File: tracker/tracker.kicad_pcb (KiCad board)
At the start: 2 copper layers, 50.5 x 56.9 mm, 76 parts, among them J1 Conn_01x10, J2 SIM_Card, M1 BG96, Q1 SSM6N7002KFU, Q2 SSM6N7002KFU, Q3 SSM6N7002KFU, U1 STM32U545CEUx, U2 GD25QxxxEY, U3 74LVC244APW,118, U4 AP22800HB-7, U5 DF5A6.8JE,LM, U6 LMR51430, U7 AP61100Z6, U8 BQ25601, Y1 32.768KHz, Y2 8MHz

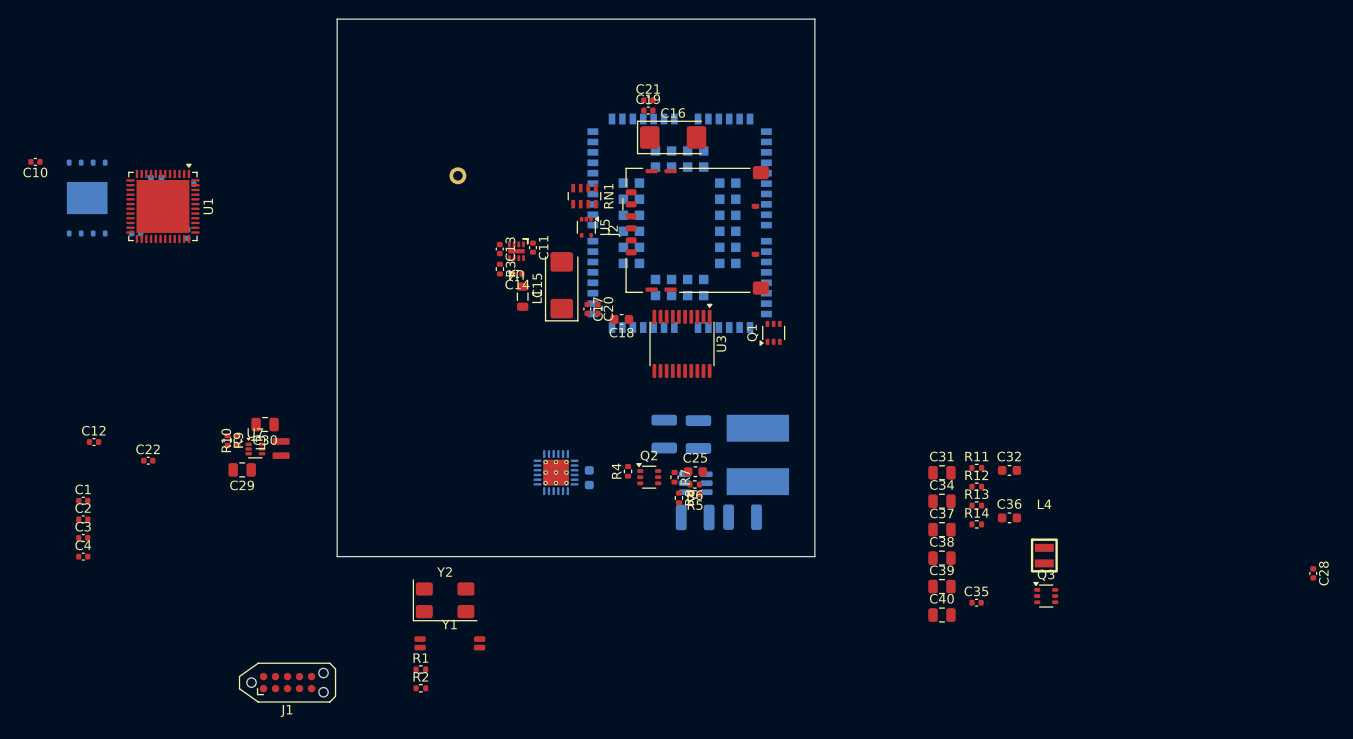
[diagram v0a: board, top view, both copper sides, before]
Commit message: save
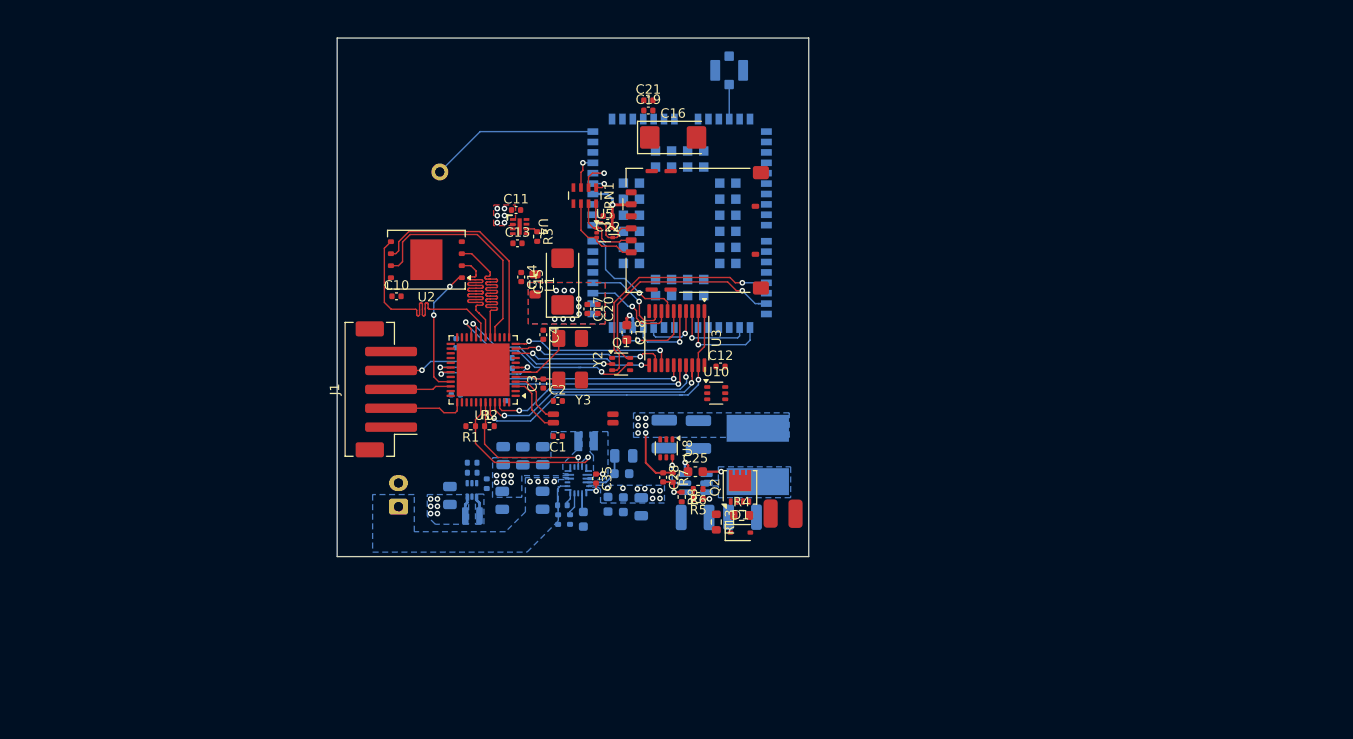
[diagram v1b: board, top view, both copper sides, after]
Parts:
- removed C34: 10u, Capacitor_SMD:C_0805_2012Metric
- removed Q3: SSM6N7002KFU, Package_TO_SOT_SMD:SOT-363_SC-70-6
- removed Y1: 32.768KHz, Crystal:Crystal_SMD_SeikoEpson_MC146-4Pin_6.7x1.5mm
- added C41: 10u, Capacitor_SMD:C_0805_2012Metric, B.Cu at (152.9, 87.2)
- added C42: 0.1u, Capacitor_SMD:C_0603_1608Metric, B.Cu at (152.7, 89.1)
- added D1: 12V, Diode_SMD:D_SOD-323, F.Cu at (165.2, 95.3)
- added J3: Conn_01x01, My Footprints:pad_smd_1.5x3, F.Cu at (168.4, 93.3)
- added J4: Conn_01x01, My Footprints:pad_smd_1.5x3, F.Cu at (171.1, 93.3)
- added J5: Conn_Coaxial, Connector_Coaxial:U.FL_Molex_MCRF_73412-0110_Vertical, B.Cu at (164.0, 46.4)
- added J6: Conn_01x02, Connector_JST:JST_XH_B2B-XH-A_1x02_P2.50mm_Vertical, B.Cu at (129.0, 92.6)
- added R15: TBD, Resistor_SMD:R_0402_1005Metric, B.Cu at (147.2, 94.0)
- added U10: PUMH10,115, Package_TO_SOT_SMD:SOT-363_SC-70-6, F.Cu at (162.7, 80.6)
- added U9: ~, My Footprints:BQ25622E, B.Cu at (148.1, 89.8)
- added Y3: 32.768KHz, Crystal:Crystal_SMD_SeikoEpson_MC146-4Pin_6.7x1.5mm, F.Cu at (148.6, 83.3)
- C29, C30, C31, C32, C36, C37, C38, C39, C40, L3, L4, R10, R11, R12, R9, U7: moved to B.Cu
- J1: value Conn_01x10 -> Conn_01x05; footprint Connector:Tag-Connect_TC2050-IDC-NL_2x05_P1.27mm_Vertical -> Connector_JST:JST_PH_B5B-PH-SM4-TB_1x05-1MP_P2.00mm_Vertical
- Q2: value SSM6N7002KFU -> DMP2008UFG; footprint Package_TO_SOT_SMD:SOT-363_SC-70-6 -> Package_SON:Diodes_PowerDI3333-8
- R13: value 37K -> 10K; footprint Resistor_SMD:R_0402_1005Metric -> Resistor_SMD:R_0603_1608Metric
- R14: value 100K -> 200K; moved to B.Cu
- R4: value 200K -> 220K; footprint Resistor_SMD:R_0402_1005Metric -> Resistor_SMD:R_0603_1608Metric
- U2: moved to F.Cu
- U8: value BQ25601 -> PUMH10,115; footprint Package_DFN_QFN:Texas_RTW_WQFN-24-1EP_4x4mm_P0.5mm_EP2.7x2.7mm_ThermalVias -> Package_TO_SOT_SMD:SOT-363_SC-70-6; moved to F.Cu
- moved C28 69.5 mm to (157.0, 89.5)
- moved C12 66.8 mm to (163.1, 77.8)
- moved C22 55.1 mm to (151.2, 61.8), turned to 180 degrees
- moved C4 54.0 mm to (144.4, 74.4), turned to -90 degrees
- moved R14 52.0 mm to (138.4, 90.2), turned to 90 degrees
- moved C2 51.8 mm to (145.9, 81.4)
- moved C3 51.4 mm to (144.4, 79.6), turned to 90 degrees
- moved C1 50.7 mm to (145.9, 85.1), turned to 180 degrees
- moved C40 49.4 mm to (140.1, 87.2), turned to 90 degrees
- moved L4 49.0 mm to (149.7, 85.7), turned to 90 degrees
- moved C39 46.5 mm to (142.2, 87.2), turned to 90 degrees
- moved C36 45.1 mm to (148.6, 93.9), turned to -90 degrees
- moved R12 44.4 mm to (145.9, 94.0), turned to -90 degrees
- moved R11 44.0 mm to (146.4, 92.4), turned to 180 degrees
- moved C38 43.6 mm to (144.3, 87.2), turned to 90 degrees
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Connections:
- net Net-(AE1-A) renamed /gsm/ANT_GNSS
- C10 pad 1: Net-(U2-VCC) -> +3V3
- C23 pad 1: /psu/+VIN -> /psu/+VIN_PROTECTED
- C24 pad 1: /psu/+VIN -> /psu/+VIN_PROTECTED
- C29 pad 1: /low_voltage_psu/+VSYS -> +VSYS
- C30 pad 1: /low_voltage_psu/+3V3 -> +3V3
- C35 pad 2: Net-(U8-BTST) -> Net-(U9-BTST)
- C36 pad 1: Net-(U8-REGN) -> Net-(U9-REGN)
- C37 pad 1: Net-(C37-Pad1) -> /battery charger/+BAT
- C38 pad 1: /battery charger/+VSYS -> +VSYS
- C39 pad 1: /battery charger/+VSYS -> +VSYS
- C40 pad 1: /battery charger/+VSYS -> +VSYS
- J1 pad 5: unconnected-(J1-Pin_5-Pad5) -> GND
- L3 pad 2: /low_voltage_psu/+3V3 -> +3V3
- L4 pad 2: /battery charger/+VSYS -> +VSYS
- M1 pad 60: unconnected-(M1-ANT_MAIN-Pad60) -> /gsm/ANT_MAIN
- Q2 pad 1: /mcu/PSU_CTRL -> /psu/+VIN_PROTECTED
- Q2 pad 2: +3V3 -> /psu/+VIN_PROTECTED
- Q2 pad 3: unconnected-(Q2B-D-Pad3) -> /psu/+VIN_PROTECTED
- Q2 pad 4: unconnected-(Q2B-S-Pad4) -> Net-(D1-A)
- Q2 pad 5: unconnected-(Q2B-G-Pad5) -> /+VIN
- R11 pad 1: Net-(U8-REGN) -> Net-(U9-TS_BIAS)
- R11 pad 2: Net-(U8-TS) -> Net-(U9-TS)
- R12 pad 1: Net-(U8-TS) -> Net-(U9-TS)
- R13 pad 1: Net-(C37-Pad1) -> Net-(D1-A)
- R13 pad 2: /battery charger/BAT_LEVEL -> GND
- R14 pad 1: /battery charger/BAT_LEVEL -> /battery charger/CHARGER_PG
- R14 pad 2: GND -> +VSYS
- R4 pad 1: +3V3 -> /psu/+VIN_PROTECTED
- R4 pad 2: /mcu/PSU_CTRL -> Net-(D1-A)
- R5 pad 1: /psu/+VIN -> /psu/+VIN_PROTECTED
- R5 pad 2: Net-(Q2A-D) -> Net-(U6-EN)
- R6 pad 2: Net-(Q2A-D) -> Net-(U6-EN)
- R9 pad 2: /low_voltage_psu/+3V3 -> +3V3
- RN1 pad 1: /gsm/SIM_CLK -> /gsm/SIM_RST
- RN1 pad 3: /gsm/SIM_RST -> /gsm/SIM_CLK
- RN1 pad 6: Net-(J2-RST) -> Net-(J2-CLK)
- RN1 pad 8: Net-(J2-CLK) -> Net-(J2-RST)
- U1 pad 14: /mcu/OCTOSPI1_NCS -> unconnected-(U1-PA4-Pad14)
- U1 pad 20: unconnected-(U1-PB2-Pad20) -> /gsm/GSM_RESET
- U1 pad 21: unconnected-(U1-PB10-Pad21) -> /gsm/GSM_PWRKEY
- U1 pad 29: /gsm/GSM_STATUS -> unconnected-(U1-PA8-Pad29)
- U1 pad 33: unconnected-(U1-PA12-Pad33) -> /mcu/OCTOSPI1_NCS
- U1 pad 34: unconnected-(U1-PA13-Pad34) -> /mcu/SWDIO
- U1 pad 37: unconnected-(U1-PA14-Pad37) -> /mcu/SWCLK
- U1 pad 42: unconnected-(U1-PB6-Pad42) -> /mcu/I2C_SCL
- U1 pad 43: unconnected-(U1-PB7-Pad43) -> /mcu/I2C_SDA
- U1 pad 44: unconnected-(U1-PH3-Pad44) -> /gsm/GSM_LINE_BUF_EN
- U1 pad 45: unconnected-(U1-PB8-Pad45) -> /gsm/GSM_AP_READY
- U1 pad 46: unconnected-(U1-PB9-Pad46) -> /gsm/GSM_STATUS
- U2 pad 8: Net-(U2-VCC) -> +3V3
- U3 pad 1: (no net) -> /gsm/GSM_LINE_BUF_EN
- U6 pad 3: /psu/+VIN -> /psu/+VIN_PROTECTED
- U6 pad 5: Net-(Q2A-D) -> Net-(U6-EN)
- U7 pad 3: /low_voltage_psu/+VSYS -> +VSYS
- U7 pad 5: /low_voltage_psu/+VSYS -> /battery charger/CHARGER_PG
- U7 pad 6: /low_voltage_psu/+3V3 -> +3V3
- U8 pad 1: +5V -> /mcu/PSU_CTRL
- U8 pad 2: GND -> +3V3
- U8 pad 3: /battery charger/CHARGER_PG -> unconnected-(U8-Pad3)
- U8 pad 4: /battery charger/CHARGER_STAT -> unconnected-(U8-Pad4)
- U8 pad 5: /battery charger/CHARGER_SCL -> unconnected-(U8-Pad5)
- U8 pad 6: /battery charger/CHARGER_SDA -> Net-(U6-EN)
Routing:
- net /gsm/GSM_LINE_BUF_EN: track 0.00 -> 33.5 mm, vias 0 -> 2
- net /gsm/GPS_TX: track 0.00 -> 28.6 mm, vias 0 -> 2
- net /gsm/GPS_RX: track 0.00 -> 27.8 mm, vias 0 -> 2
- net /gsm/GSM_AP_READY: track 0.00 -> 26.6 mm, vias 0 -> 2
- net /gsm/PWRKEY: track 0.00 -> 25.4 mm, vias 0 -> 1
- net /gsm/RESET: track 0.00 -> 25.0 mm, vias 0 -> 1
- net /mcu/OCTOSPI1_IO0: track 0.00 -> 24.3 mm
- net /mcu/OCTOSPI1_IO2: track 0.00 -> 24.1 mm
- net /mcu/OCTOSPI1_IO1: track 0.00 -> 24.1 mm
- net /mcu/OCTOSPI1_IO3: track 0.00 -> 24.1 mm
- net /gsm/GSM_STATUS: track 0.00 -> 23.6 mm, vias 0 -> 2
- net /mcu/OCTOSPI1_CLK: track 0.00 -> 23.4 mm
- net /gsm/GSM_PWRKEY: track 0.00 -> 23.2 mm, vias 0 -> 2
- net /mcu/I2C_SCL: track 0.00 -> 19.1 mm, vias 0 -> 1
- net /gsm/GSM_RESET: track 0.00 -> 18.0 mm, vias 0 -> 2
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- added copper zone on B.Cu, net +3V3
- added copper zone on In1.Cu, net +3V3
- added copper zone on B.Cu, net +5V
- added copper zone on In1.Cu, net +5V
- added copper zone on B.Cu, net +VSYS
- added copper zone on F.Cu, net +VSYS
- added copper zone on In1.Cu, net +VSYS
- added copper zone on B.Cu, net /battery charger/+BAT
- added copper zone on In1.Cu, net /battery charger/+BAT
- added copper zone on B.Cu, net /battery charger/BQ_SW
- added copper zone on B.Cu, net /gsm/+VBAT_GSM
- added copper zone on F.Cu, net /gsm/+VBAT_GSM
- added copper zone on B.Cu, net Net-(U6-SW)
- added copper zone on B.Cu, net Net-(U7-SW)
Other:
- board size 50.5 x 56.9 mm -> 49.9 x 54.9 mm
- copper layers 2 -> 4
